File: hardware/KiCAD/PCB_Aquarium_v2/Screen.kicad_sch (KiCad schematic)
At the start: 6 parts, among them J25 Conn_01x04, J26 Conn_01x04, J27 Conn_01x04, J28 Conn_01x04, J29 Conn_01x04, J30 Conn_01x04

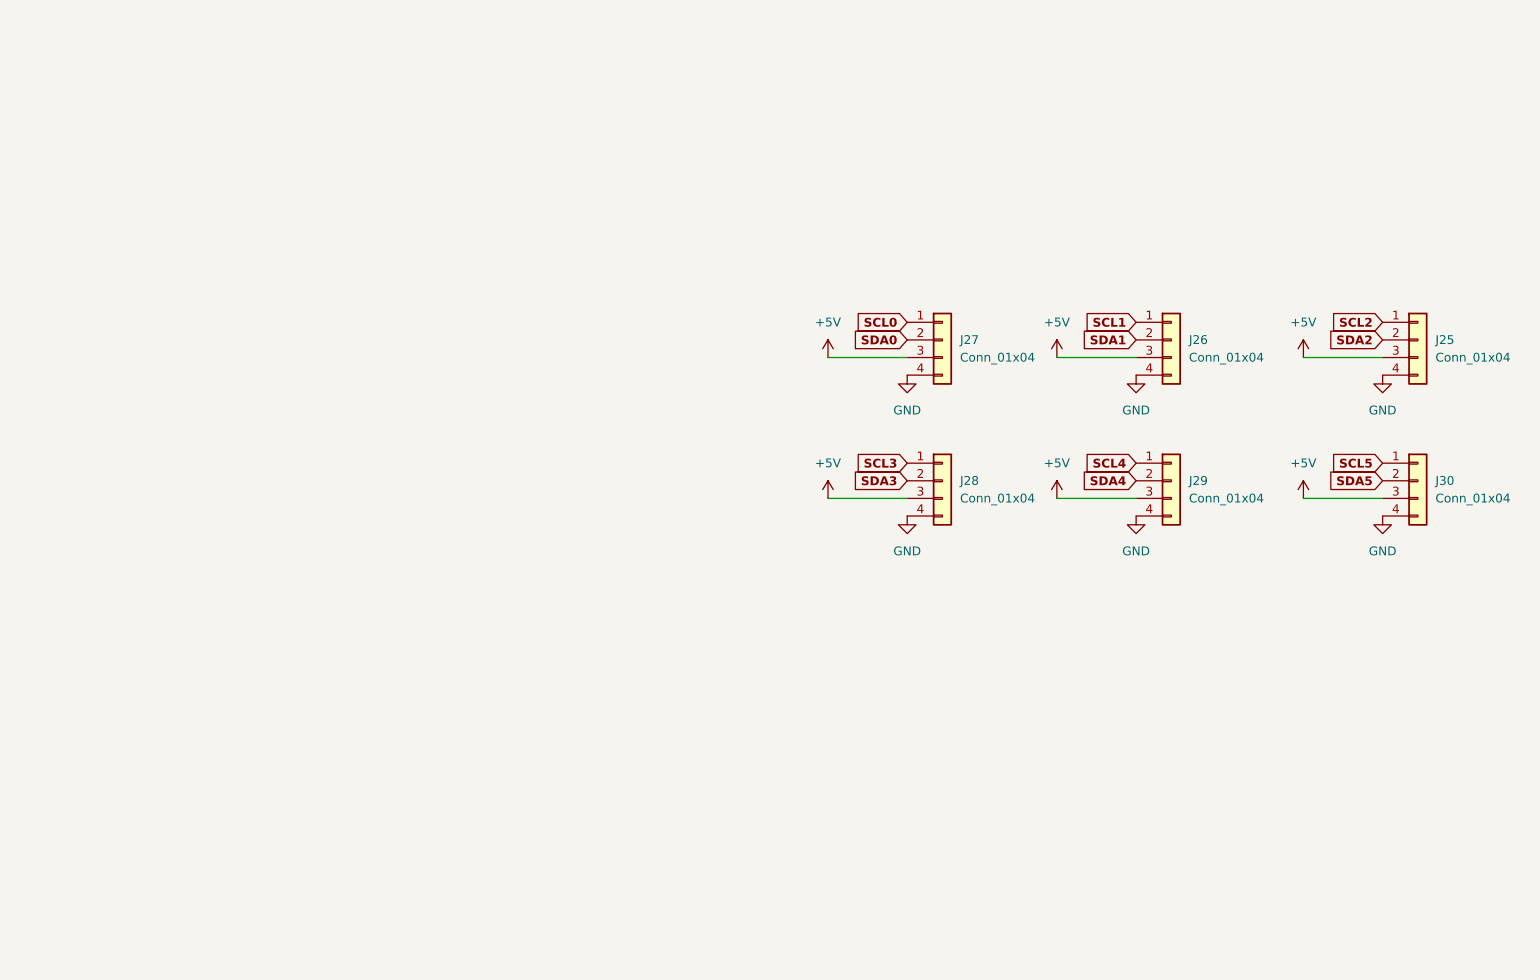
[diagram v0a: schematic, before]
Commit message: PCB principal finis
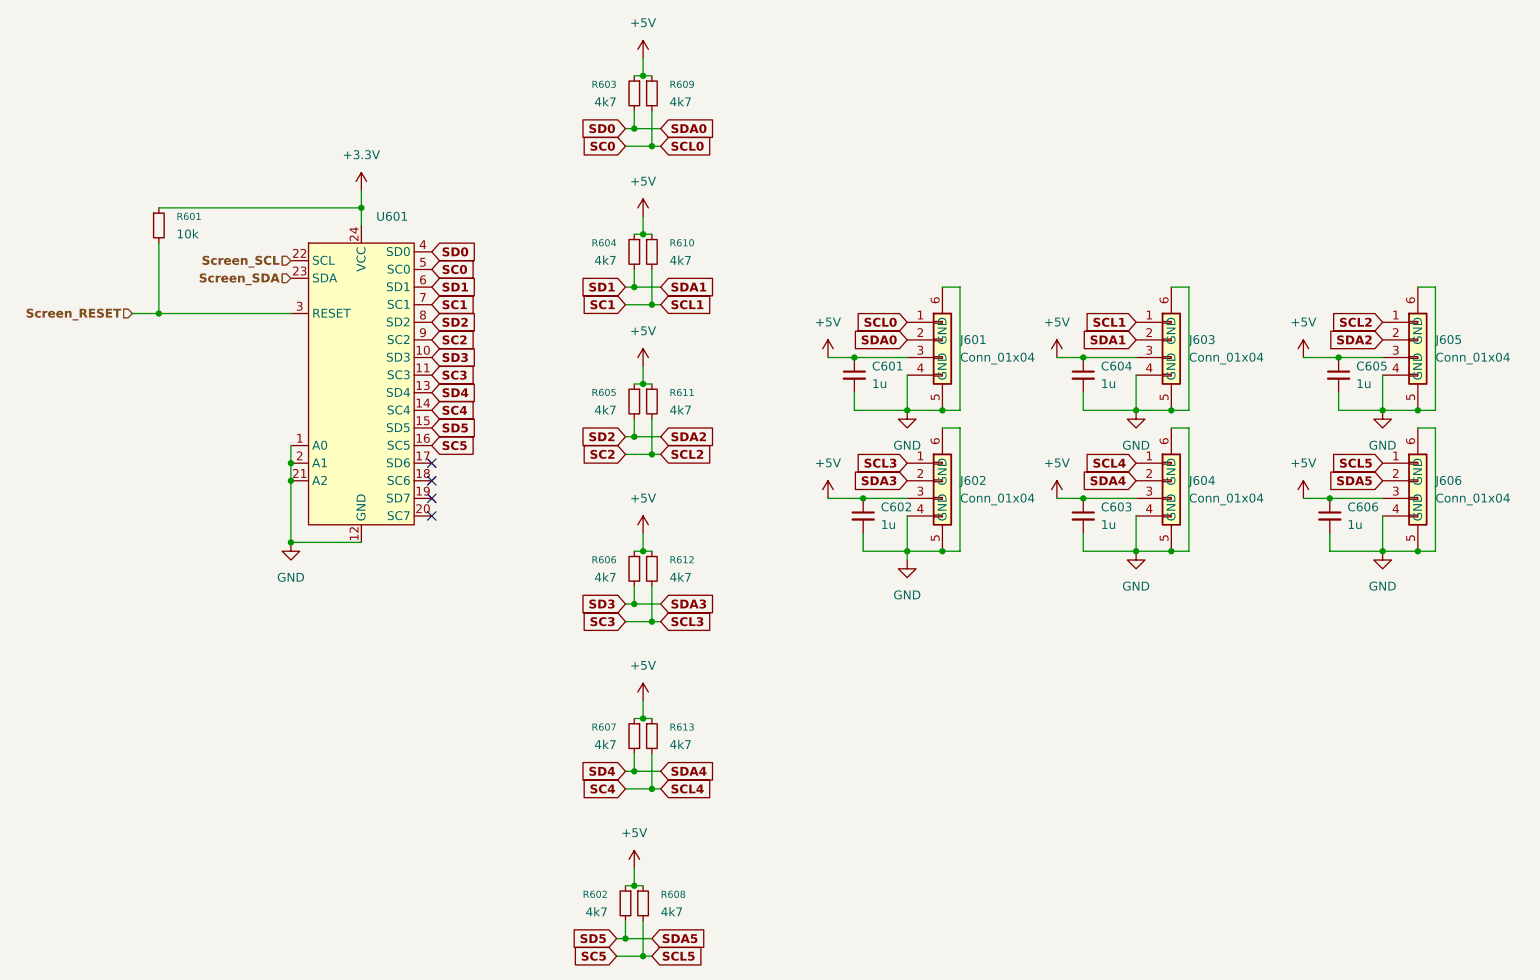
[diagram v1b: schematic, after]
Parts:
- added C601, C602, C603, C604, C605, C606: 1u, Capacitor_SMD:C_0603_1608Metric, symbol Device:C_Small
- added R601: 10k, Resistor_SMD:R_0402_1005Metric, symbol Device:R_Small
- added R602, R603, R604, R605, R606, R607, R608, R609, R610, R611, R612, R613: 4k7, Resistor_SMD:R_0201_0603Metric, symbol Device:R_Small
- added U601: ~, Package_SO:TSSOP-24_4.4x7.8mm_P0.65mm, symbol my_lib:PI4MSD5V9547
- J601: renamed from J27; footprint (none) -> mylib:Wurth_Vertical_4_pos_0.8mm; symbol Connector_Generic:Conn_01x04 -> my_lib:JST_SH_4_Vertical
- J602: renamed from J28; footprint (none) -> mylib:Wurth_Vertical_4_pos_0.8mm; symbol Connector_Generic:Conn_01x04 -> my_lib:JST_SH_4_Vertical
- J603: renamed from J26; footprint (none) -> mylib:Wurth_Vertical_4_pos_0.8mm; symbol Connector_Generic:Conn_01x04 -> my_lib:JST_SH_4_Vertical
- J604: renamed from J29; footprint (none) -> mylib:Wurth_Vertical_4_pos_0.8mm; symbol Connector_Generic:Conn_01x04 -> my_lib:JST_SH_4_Vertical
- J605: renamed from J25; footprint (none) -> mylib:Wurth_Vertical_4_pos_0.8mm; symbol Connector_Generic:Conn_01x04 -> my_lib:JST_SH_4_Vertical
- J606: renamed from J30; footprint (none) -> mylib:Wurth_Vertical_4_pos_0.8mm; symbol Connector_Generic:Conn_01x04 -> my_lib:JST_SH_4_Vertical
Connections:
- net +5V: now also C601.1, C602.1, C603.1, C604.1, C605.1, C606.1, R602.1, R603.1, R604.1, R605.1, R606.1, R607.1, R608.1, R609.1, R610.1, R611.1, R612.1, R613.1
- net GND: now also J601.5 (GND), J601.6 (GND), J602.5 (GND), J602.6 (GND), J603.5 (GND), J603.6 (GND), J604.5 (GND), J604.6 (GND), J605.5 (GND), J605.6 (GND), J606.5 (GND), J606.6 (GND), C601.2, C602.2, C603.2, C604.2, C605.2, C606.2, U601.1 (A0), U601.12 (GND), U601.2 (A1), U601.21 (A2)
- net SCL0 renamed SC0
- net SC0: now also R609.2, U601.5 (SC0)
- net SCL1 renamed SC1
- net SC1: now also R610.2, U601.7 (SC1)
- net SCL2 renamed SC2
- net SC2: now also R611.2, U601.9 (SC2)
- net SCL3 renamed SC3
- net SC3: now also R612.2, U601.11 (SC3)
- net SCL4 renamed SC4
- net SC4: now also R613.2, U601.14 (SC4)
- net SCL5 renamed SC5
- net SC5: now also R608.2, U601.16 (SC5)
- net SDA0 renamed SD0
- net SD0: now also R603.2, U601.4 (SD0)
- net SDA1 renamed SD1
- net SD1: now also R604.2, U601.6 (SD1)
- net SDA2 renamed SD2
- net SD2: now also R605.2, U601.8 (SD2)
- net SDA3 renamed SD3
- net SD3: now also R606.2, U601.10 (SD3)
- net SDA4 renamed SD4
- net SD4: now also R607.2, U601.13 (SD4)
- net SDA5 renamed SD5
- net SD5: now also R602.2, U601.15 (SD5)
- new net +3.3V: R601.1, U601.24 (VCC)
- new net Screen_RESET: R601.2, U601.3 (RESET)
- new net Screen_SCL: U601.22 (SCL)
- new net Screen_SDA: U601.23 (SDA)
- no-connect marks 0 -> 4
